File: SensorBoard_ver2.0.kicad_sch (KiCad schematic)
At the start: 58 parts, among them J1 CANConn, J10 USB_C, J13 Abso, J14 Abso, J15 STLink, J16 Abso, J18 Abso, J19 Abso, J2 CANConn, J20 Enc5, J3 Enc1, J4 Enc2, J5 Enc3, J6 Enc4, SW1 CAN_Terminal, SW2 IDSetSW, SW3 Reset, SW4 IDSetSW, SW5 Terminal, U1 L7805, U2 ATA6561, U3 3.3V Regulator, U4 STM32F303K8Tx, U5 MAX3485, Y1 Crystal

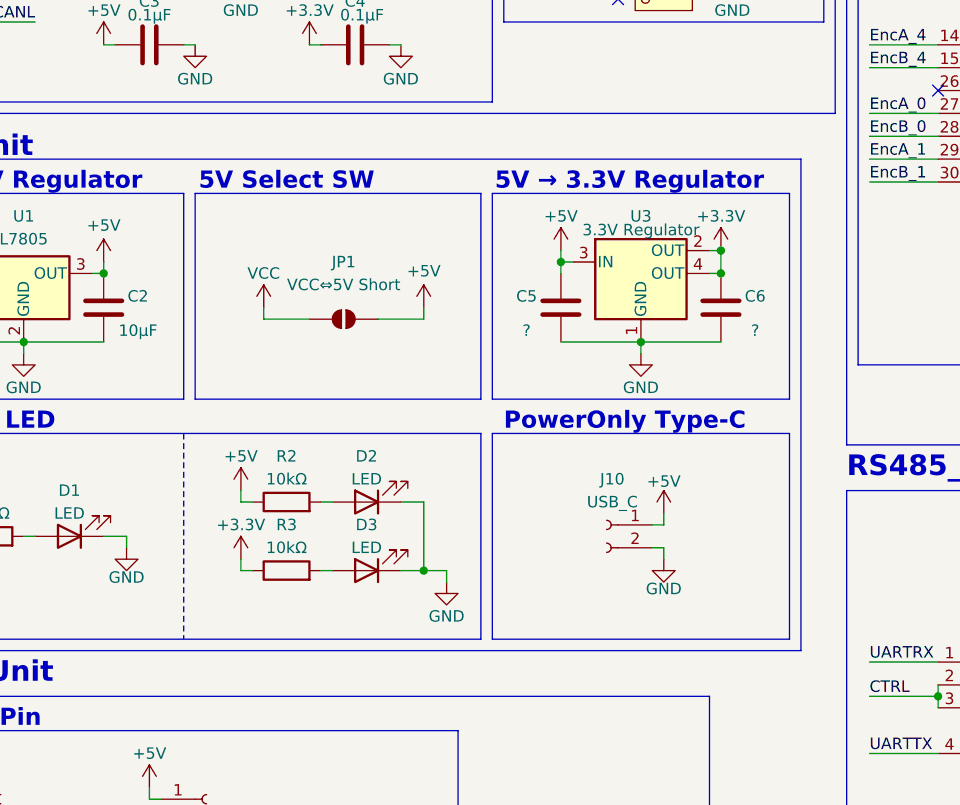
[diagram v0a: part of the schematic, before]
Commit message: 大改造する前のバックアップ
大改造して、失敗したときのバックアップです
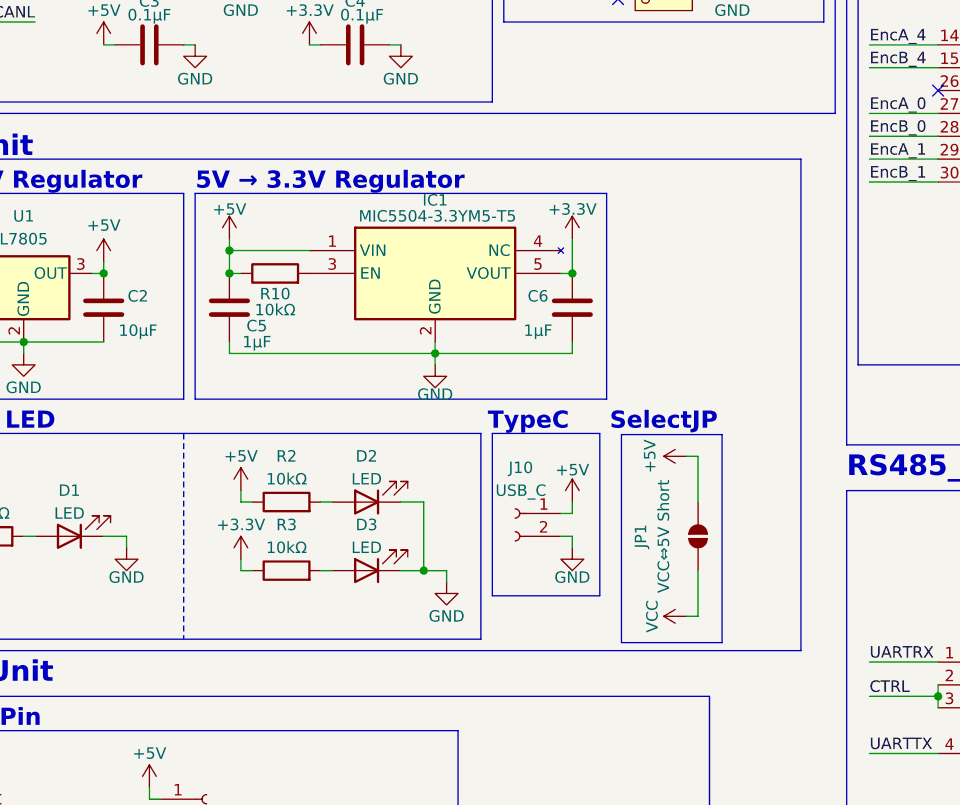
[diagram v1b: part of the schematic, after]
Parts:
- removed U3: 3.3V Regulator, Package_TO_SOT_SMD:SOT-223, symbol Regulator_Linear:L7805
- added IC1: MIC5504-3.3YM5-T5, SOT95P280X130-5N, symbol MIC5504-3_3YM5-T5:MIC5504-3.3YM5-T5
- added R10: 10kΩ, Resistor_SMD:R_0603_1608Metric, symbol Device:R
- C5, C6: value ? -> 1μF
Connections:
- net +3.3V: now also IC1.5 (VOUT)
- net +5V: now also IC1.1 (VIN), R10.1
- net GND: now also IC1.2 (GND)
- new net: IC1.3 (EN), R10.2
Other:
- note added: "SelectJP"
- note added: "TypeC"
- note removed: "5V Select SW"
- note removed: "PowerOnly Type-C"
- moved on the sheet: J10, JP1

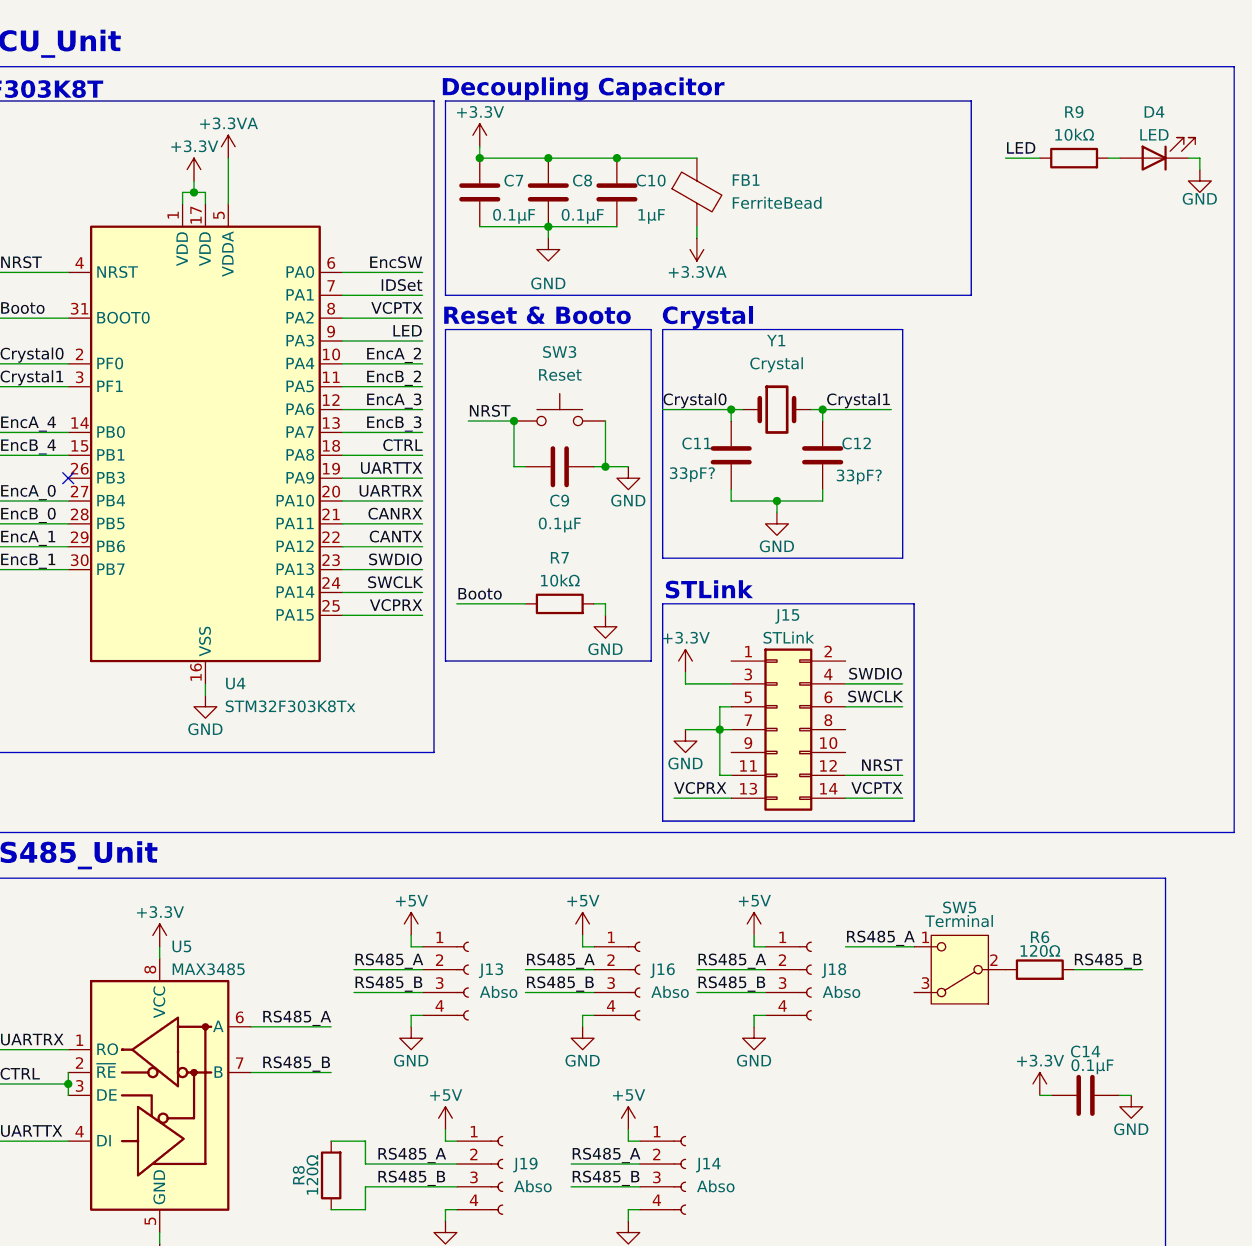
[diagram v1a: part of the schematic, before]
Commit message: 大改造したあと　ver01
特になし、アップロードしたファイル間違えてるかもしれないくらい？
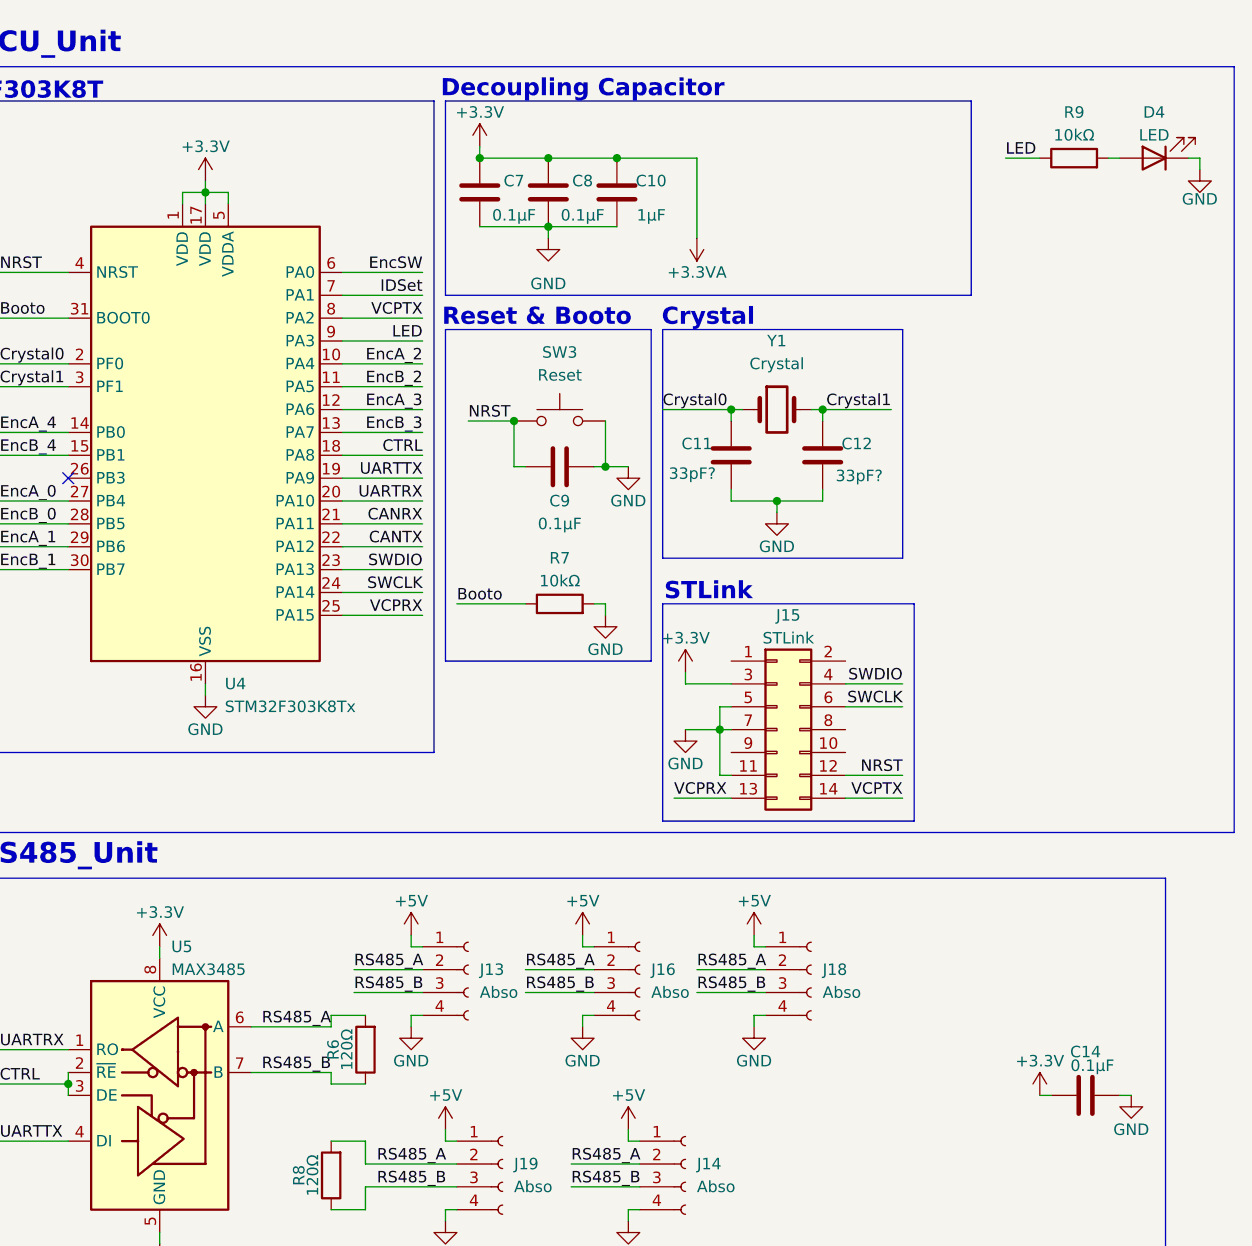
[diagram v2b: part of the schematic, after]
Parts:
- removed FB1: FerriteBead, Inductor_SMD:L_0603_1608Metric, symbol Device:FerriteBead
- removed SW5: Terminal, Connector_PinHeader_2.54mm:PinHeader_1x03_P2.54mm_Vertical, symbol Switch:SW_Nidec_CAS-120A1
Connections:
- net +3.3VA is gone; now on net +3.3V: U4.5 (VDDA)
- net RS485_A: now also R6.2
- net RS485_B: now also R6.1; no longer R6.2
